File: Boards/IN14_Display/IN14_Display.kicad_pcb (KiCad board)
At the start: 2 copper layers, 160 x 50 mm, 49 parts, among them IC1 TPIC6B596DW, IC2 TPIC6B596DW, IC3 TPIC6B596DW, IC4 TPIC6B596DW, IC5 TPIC6B596DW, IC6 TPIC6B596DW, IC7 TPIC6B596DW, IC8 TPIC6B596DW, P1 CONN_01X02, P2 CONN_01X06, Q1 BC817

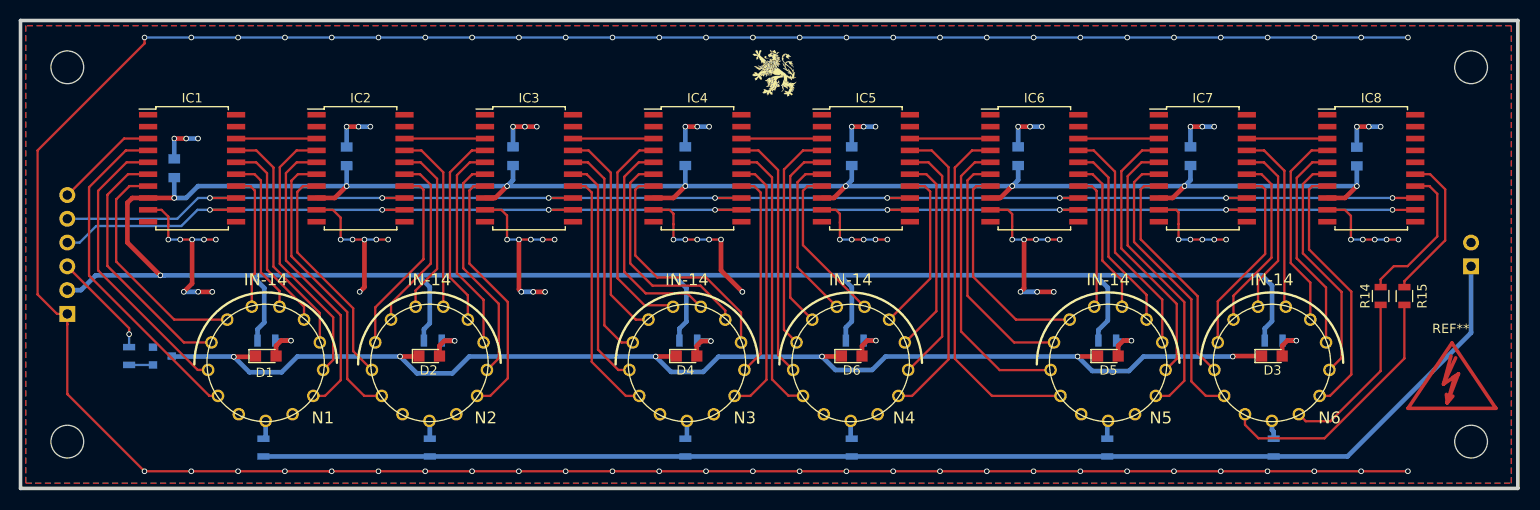
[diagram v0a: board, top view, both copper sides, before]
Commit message: Layout done, before PCB order
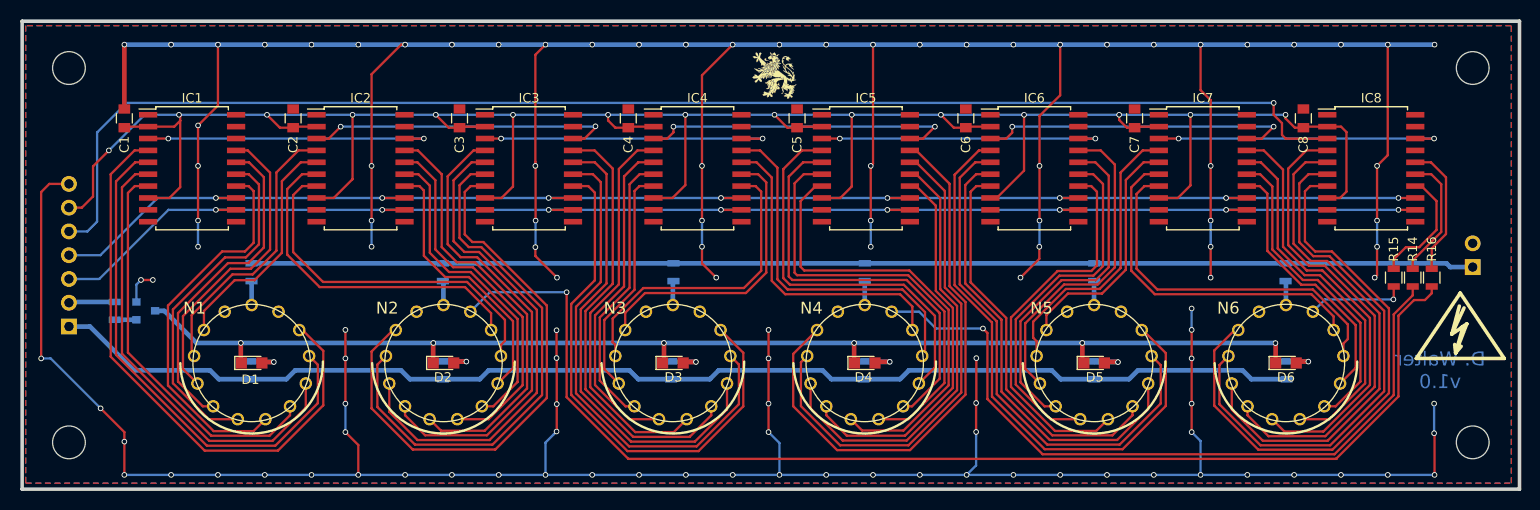
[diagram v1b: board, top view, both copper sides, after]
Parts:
- removed P2: CONN_01X06, Pin_Headers:Pin_Header_Straight_1x06_Pitch2.54mm
- removed the REF** at (216.5, 110.5)
- added J1: Conn_01x07, Pin_Headers:Pin_Header_Straight_1x07_Pitch2.54mm, B.Cu at (68.8, 104.5)
- added R16: 16k, Resistors_SMD:R_0805, F.Cu at (214.4, 99.3)
- added REF**: Symbol_HighVoltage_Type2_CopperTop_VerySmall, MySymbols:Symbol_HighVoltage_Type2_SilkTop_VerySmall, F.Cu at (217.4, 105.2)
- C1, C2, C3, C4, C5, C6, C7, C8: moved to F.Cu
- moved C2 96.0 mm to (92.7, 82.3)
- moved C7 66.5 mm to (182.6, 82.3)
- moved R9 64.5 mm to (133.1, 109.2), turned to 90 degrees
- moved D3 64.0 mm to (133.3, 108.4)
- moved C4 48.8 mm to (128.5, 82.3)
- moved D6 46.4 mm to (198.8, 108.4)
- moved R12 46.3 mm to (198.9, 109.2), turned to 90 degrees
- moved C3 24.5 mm to (110.5, 82.3)
- moved C1 24.1 mm to (74.7, 82.3)
- moved C5 24.0 mm to (146.6, 82.3)
- moved D4 19.1 mm to (153.8, 108.4)
- moved R10 19.0 mm to (153.7, 109.2), turned to 90 degrees
- moved R2 18.8 mm to (108.7, 98.7), turned to 270 degrees
- moved R5 18.8 mm to (178.3, 98.7), turned to 270 degrees
- moved R4 18.8 mm to (153.8, 98.7), turned to 270 degrees
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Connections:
- IC1 pad 10: (no net) -> GND
- IC1 pad 11: (no net) -> GND
- IC1 pad 18: Net-(IC1-Pad18) -> (no net)
- IC1 pad 19: (no net) -> GND
- IC1 pad 2: (no net) -> VCC
- IC2 pad 10: (no net) -> GND
- IC2 pad 11: (no net) -> GND
- IC2 pad 18: Net-(IC2-Pad18) -> Net-(IC1-Pad3)
- IC2 pad 19: (no net) -> GND
- IC2 pad 2: (no net) -> VCC
- IC2 pad 3: Net-(IC1-Pad18) -> Net-(IC2-Pad3)
- IC3 pad 10: (no net) -> GND
- IC3 pad 11: (no net) -> GND
- IC3 pad 18: Net-(IC3-Pad18) -> Net-(IC2-Pad3)
- IC3 pad 19: (no net) -> GND
- IC3 pad 2: (no net) -> VCC
- IC3 pad 3: Net-(IC2-Pad18) -> Net-(IC3-Pad3)
- IC4 pad 10: (no net) -> GND
- IC4 pad 11: (no net) -> GND
- IC4 pad 18: Net-(IC4-Pad18) -> Net-(IC3-Pad3)
- IC4 pad 19: (no net) -> GND
- IC4 pad 2: (no net) -> VCC
- IC4 pad 3: Net-(IC3-Pad18) -> Net-(IC4-Pad3)
- IC5 pad 10: (no net) -> GND
- IC5 pad 11: (no net) -> GND
- IC5 pad 18: Net-(IC5-Pad18) -> Net-(IC4-Pad3)
- IC5 pad 19: (no net) -> GND
- IC5 pad 2: (no net) -> VCC
- IC5 pad 3: Net-(IC4-Pad18) -> Net-(IC5-Pad3)
- IC6 pad 10: (no net) -> GND
- IC6 pad 11: (no net) -> GND
- IC6 pad 18: Net-(IC6-Pad18) -> Net-(IC5-Pad3)
- IC6 pad 19: (no net) -> GND
- IC6 pad 2: (no net) -> VCC
- IC6 pad 3: Net-(IC5-Pad18) -> Net-(IC6-Pad3)
- IC7 pad 10: (no net) -> GND
- IC7 pad 11: (no net) -> GND
- IC7 pad 18: Net-(IC7-Pad18) -> Net-(IC6-Pad3)
- IC7 pad 19: (no net) -> GND
- IC7 pad 2: (no net) -> VCC
- IC7 pad 3: Net-(IC6-Pad18) -> Net-(IC7-Pad3)
- IC8 pad 10: (no net) -> GND
- IC8 pad 11: (no net) -> GND
- IC8 pad 16: (no net) -> Net-(IC8-Pad16)
- IC8 pad 18: (no net) -> Net-(IC7-Pad3)
- IC8 pad 19: (no net) -> GND
- IC8 pad 2: (no net) -> VCC
- IC8 pad 3: Net-(IC7-Pad18) -> Net-(IC8-Pad3)
- N2 pad RHDP: (no net) -> Net-(N2-PadRHDP)
- N4 pad RHDP: (no net) -> Net-(N4-PadRHDP)
- N6 pad LHDP: Net-(N6-PadLHDP) -> (no net)
- R10 pad 1: VCC -> +12V
- R11 pad 1: VCC -> +12V
- R12 pad 1: VCC -> +12V
- R14 pad 1: Net-(N6-PadLHDP) -> Net-(IC8-Pad15)
- R14 pad 2: Net-(IC8-Pad14) -> Net-(N4-PadRHDP)
- R15 pad 1: Net-(N6-PadRHDP) -> Net-(IC8-Pad14)
- R15 pad 2: Net-(IC8-Pad15) -> Net-(N6-PadRHDP)
- R7 pad 1: VCC -> +12V
- R8 pad 1: VCC -> +12V
- R9 pad 1: VCC -> +12V
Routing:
- net Net-(IC8-Pad3): track 0.00 -> 148.8 mm, vias 0 -> 1
- net +12V: track 0.00 -> 136.4 mm
- net Net-(N2-PadRHDP): track 0.00 -> 130.7 mm, vias 0 -> 1
- net GND: track 483.4 -> 613.4 mm, vias 131 -> 115
- net VCC: track 356.6 -> 273.7 mm, vias 9 -> 15
- net Net-(N4-PadRHDP): track 0.00 -> 79.2 mm, vias 0 -> 1
- net Net-(IC6-Pad3): track 0.00 -> 34.6 mm, vias 0 -> 2
- net Net-(IC4-Pad3): track 0.00 -> 34.2 mm, vias 0 -> 2
- net Net-(IC3-Pad7): track 27.7 -> 61.2 mm
- net Net-(IC2-Pad3): track 0.00 -> 33.4 mm, vias 0 -> 2
- net Net-(IC8-Pad7): track 28.1 -> 61.4 mm
- net Net-(IC8-Pad6): track 25.2 -> 57.8 mm
- net Net-(IC3-Pad6): track 24.8 -> 57.4 mm
- net Net-(IC3-Pad3): track 0.00 -> 31.9 mm, vias 0 -> 2
- net Net-(IC7-Pad3): track 0.00 -> 31.4 mm, vias 0 -> 2
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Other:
- board text added: "D. Walter v1.0"
- board text added: "IN14 Display Board"
